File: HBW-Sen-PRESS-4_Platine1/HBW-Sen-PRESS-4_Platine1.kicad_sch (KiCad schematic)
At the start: 40 parts, among them IC1 MC34063AD, IC2 MAX487E, IC3 ATmega328P-A, J1 Nano_Conn, J2 Sensor_Conn, J3 RS485_Conn, J4 24V_Terminal, J5 BUS_Terminal, J6 AVR-ISP-6, Y1 16Mhz

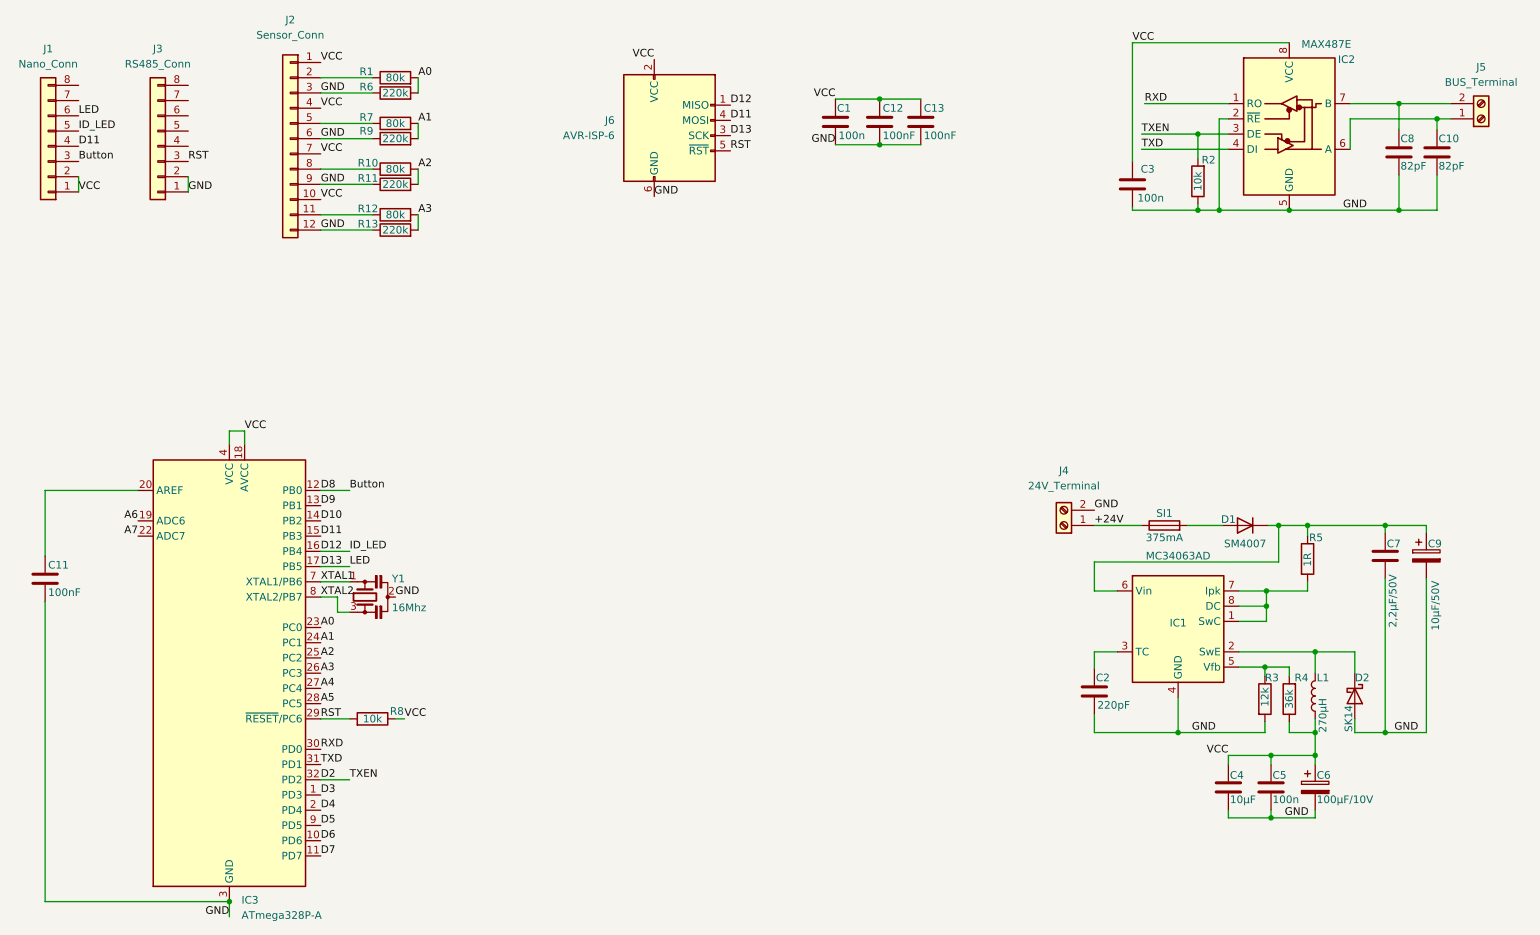
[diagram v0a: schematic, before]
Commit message: Add files via upload
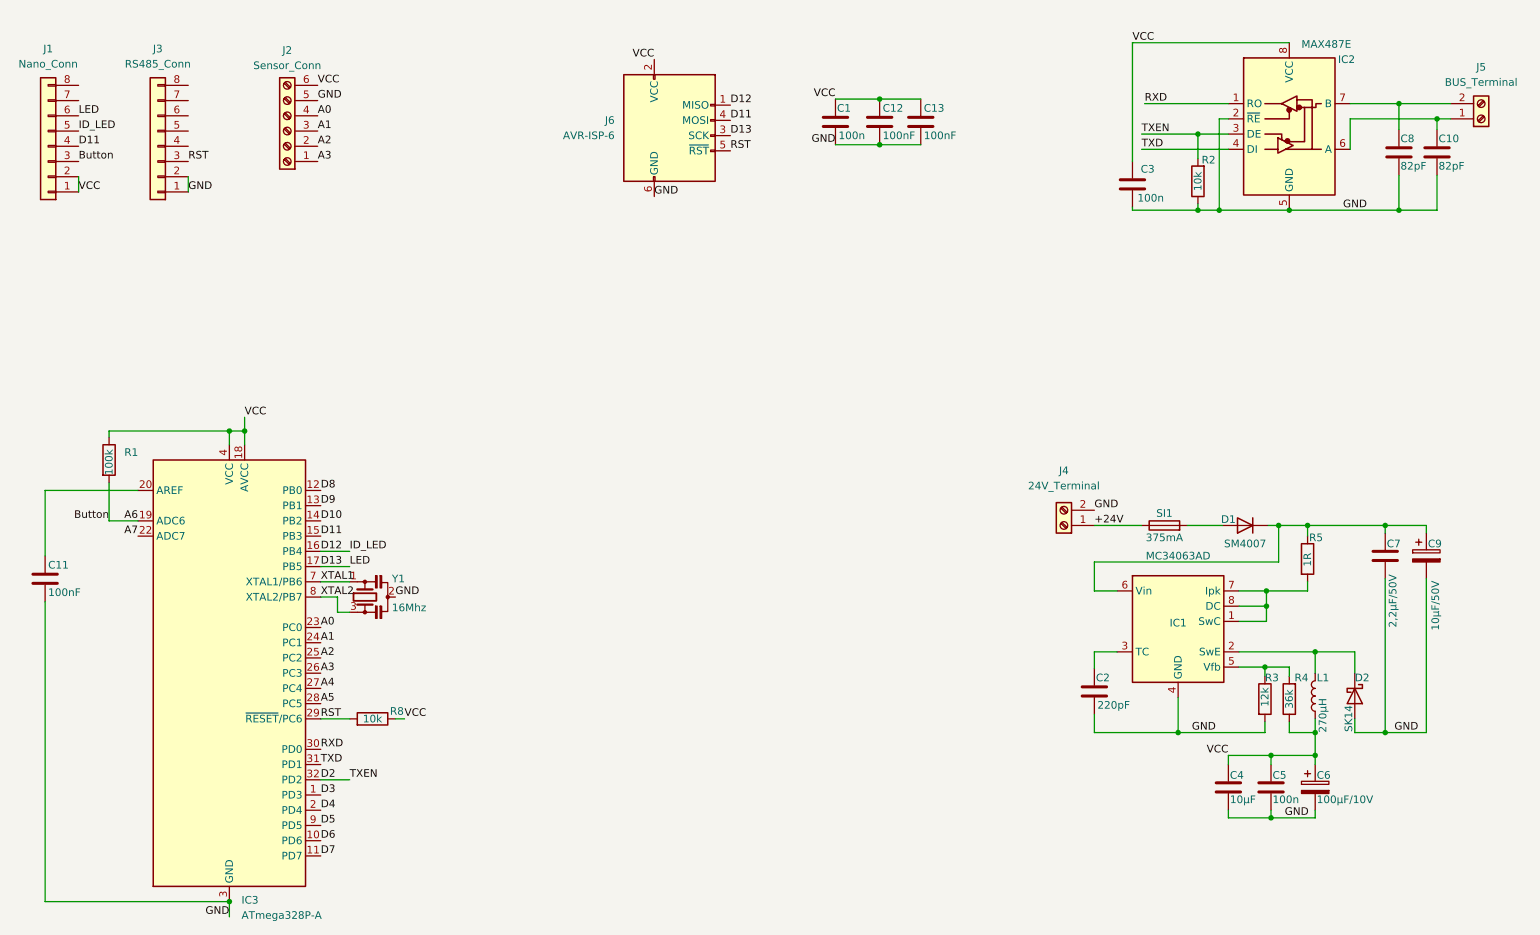
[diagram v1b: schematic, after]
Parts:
- removed J2: Sensor_Conn, Connector_PinHeader_2.54mm:PinHeader_1x12_P2.54mm_Vertical, symbol Connector_Generic:Conn_01x12
- removed R10, R12, R7: 80k, Resistor_SMD:R_0805_2012Metric_Pad1.20x1.40mm_HandSolder, symbol Device:R
- removed R11, R13, R6, R9: 220k, Resistor_SMD:R_0805_2012Metric_Pad1.20x1.40mm_HandSolder, symbol Device:R
- added J2: Sensor_Conn, TerminalBlock_CUI:TerminalBlock_CUI_TB007-508-06_1x06_P5.08mm_Horizontal, symbol Connector:Screw_Terminal_01x06
- R1: value 80k -> 100k
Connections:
- net A0: now also J2.4 (Pin_4); no longer R1.2
- net A1: now also J2.3 (Pin_3)
- net A2: now also J2.2 (Pin_2)
- net A3: now also J2.1 (Pin_1)
- net A6: now also J1.3 (Pin_3), R1.2
- net GND: now also J2.5 (Pin_5)
- net VCC: now also R1.1, J2.6 (Pin_6)
- net Button renamed D8
- net D8: no longer J1.3 (Pin_3)
